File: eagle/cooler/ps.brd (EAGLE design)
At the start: 160 x 100 mm, 18 parts, among them IC5 7812TV, J1 PIN2F061.100, J2 PIN2F061.100, J3 PIN2F061.100, J4 PIN2F061.100, J5 PIN2F061.100, J6 PIN2F061.100, Q1 2N5883, T1 2N3055, T2 2N3055

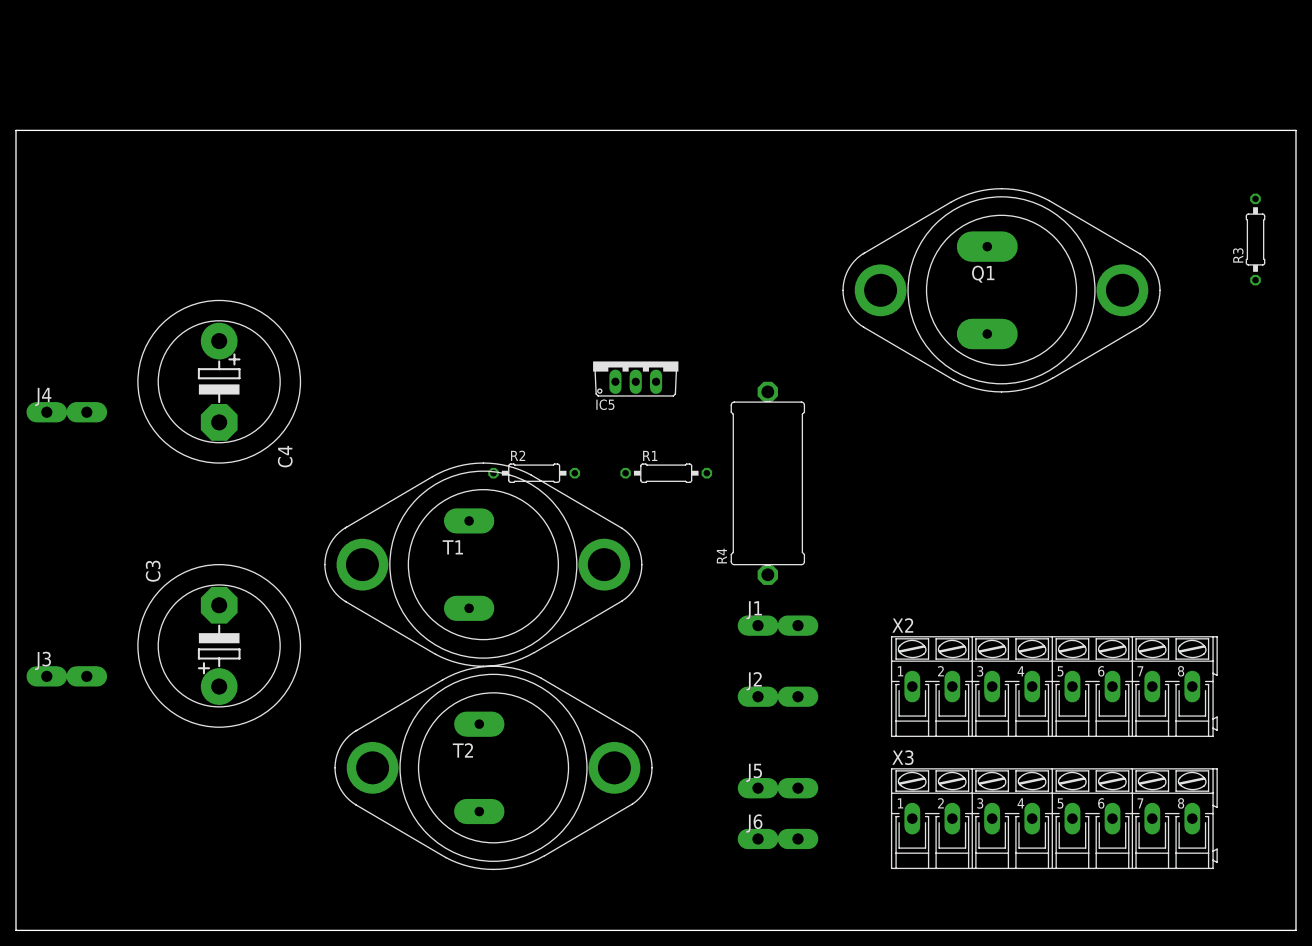
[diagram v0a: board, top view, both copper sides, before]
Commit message: layouts
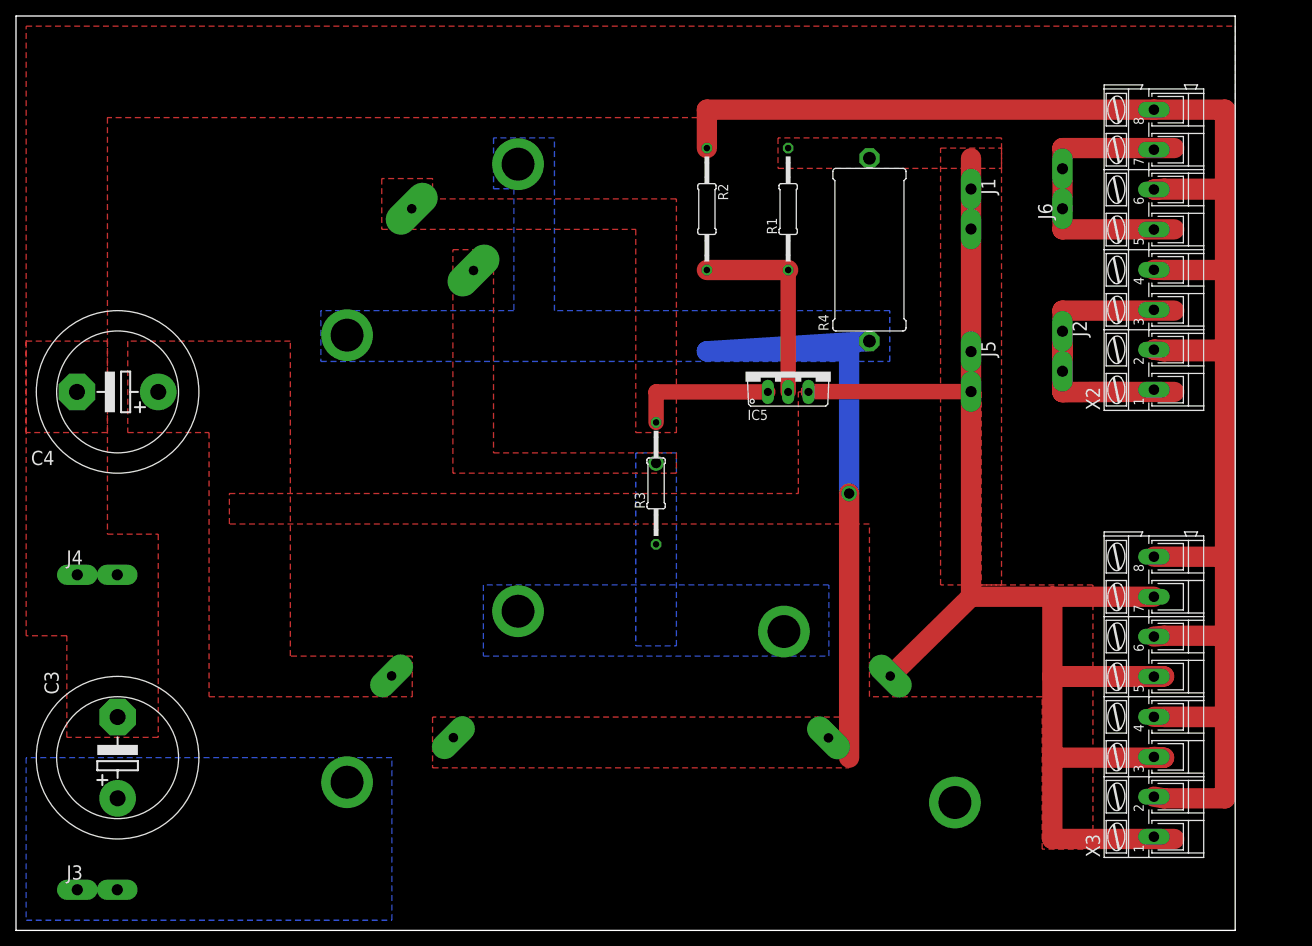
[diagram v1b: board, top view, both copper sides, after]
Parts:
- R1, R2, R3: device rcl:0207/10 -> rcl:0207/15
- moved J6 88.7 mm to (130.8, 92.7), turned to 90 degrees
- moved R3 80.9 mm to (80.0, 55.9)
- moved Q1 71.3 mm to (52.1, 85.1), flipped to the bottom, turned to 315 degrees
- moved J1 57.4 mm to (119.4, 90.2), turned to 270 degrees
- moved J5 57.4 mm to (119.4, 69.8), turned to 270 degrees
- moved X2 56.1 mm to (142.2, 85.1), turned to 90 degrees
- moved J2 55.9 mm to (130.8, 72.4), turned to 270 degrees
- moved T2 47.4 mm to (106.7, 26.7), flipped to the bottom, turned to 225 degrees
- moved R2 39.5 mm to (86.4, 90.2), turned to 270 degrees
- moved R1 36.4 mm to (96.5, 90.2), turned to 90 degrees
- moved R4 31.9 mm to (106.7, 85.1)
- moved J3 26.9 mm to (10.2, 5.08)
- moved J4 20.7 mm to (10.2, 44.5)
- moved X3 19.8 mm to (142.2, 29.2), turned to 90 degrees
- moved IC5 19.1 mm to (96.5, 69.8)
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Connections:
- removed net N$2: R4.2
- net TEC1: now also X2.1, X2.3
- net TEC2: now also X2.5
- net VDD: now also R4.2
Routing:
- net GND: track 0.00 -> 243.4 mm
- net VDD: track 0.00 -> 200.9 mm
- net N$1: track 0.00 -> 88.9 mm, vias 0 -> 1
- net TEC1: track 0.00 -> 58.3 mm
- net TEC2: track 0.00 -> 38.1 mm
- net N$5: track 0.00 -> 25.4 mm
- net N$4: track 0.00 -> 17.8 mm
- added copper zone on layer 1, net GND
- added copper zone on layer 1, net N$1
- added copper zone on layer 16, net N$1
- added copper zone on layer 1, net N$4
- added copper zone on layer 1, net VDD
- added copper zone on layer 1, net VIN
- added copper zone on layer 16, net VIN
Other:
- board size 160 x 100 mm -> 152.4 x 114.3 mm
